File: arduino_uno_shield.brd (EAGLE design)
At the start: 53 x 59.7 mm, 18 parts

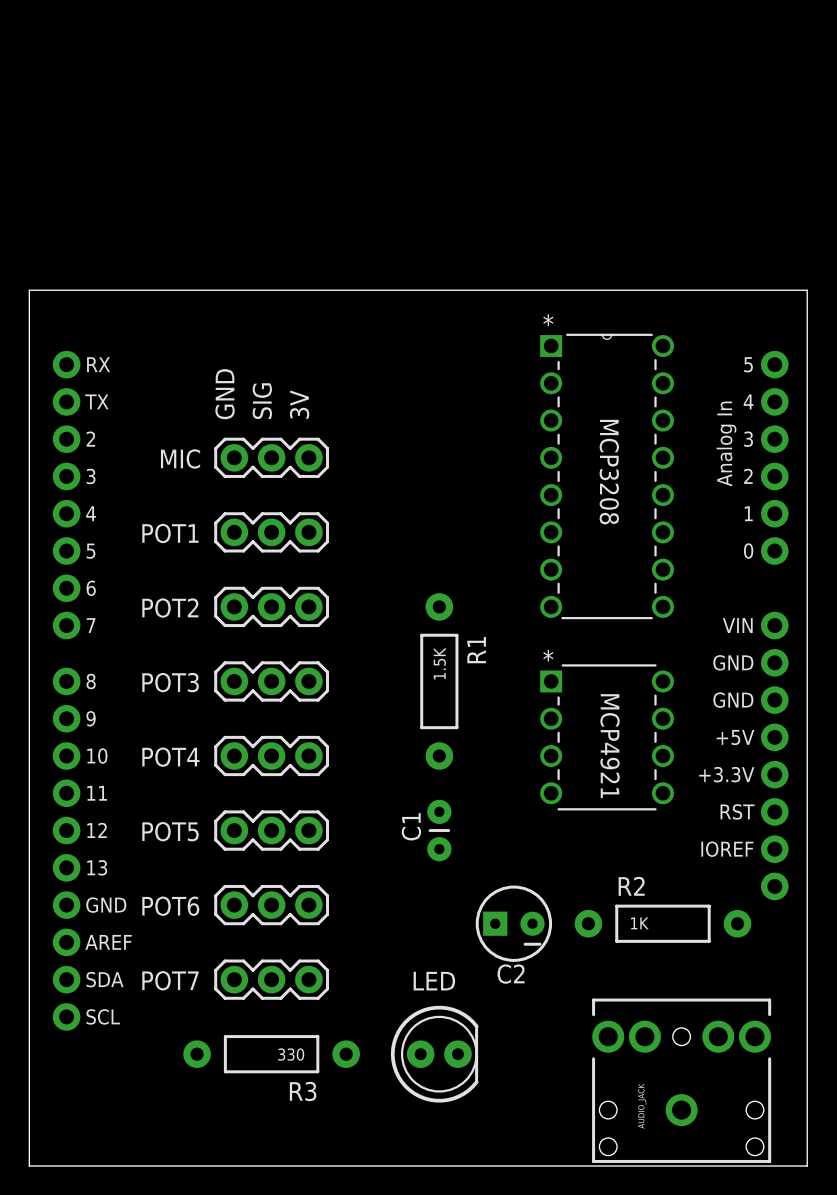
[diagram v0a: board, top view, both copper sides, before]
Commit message: created board from scratch
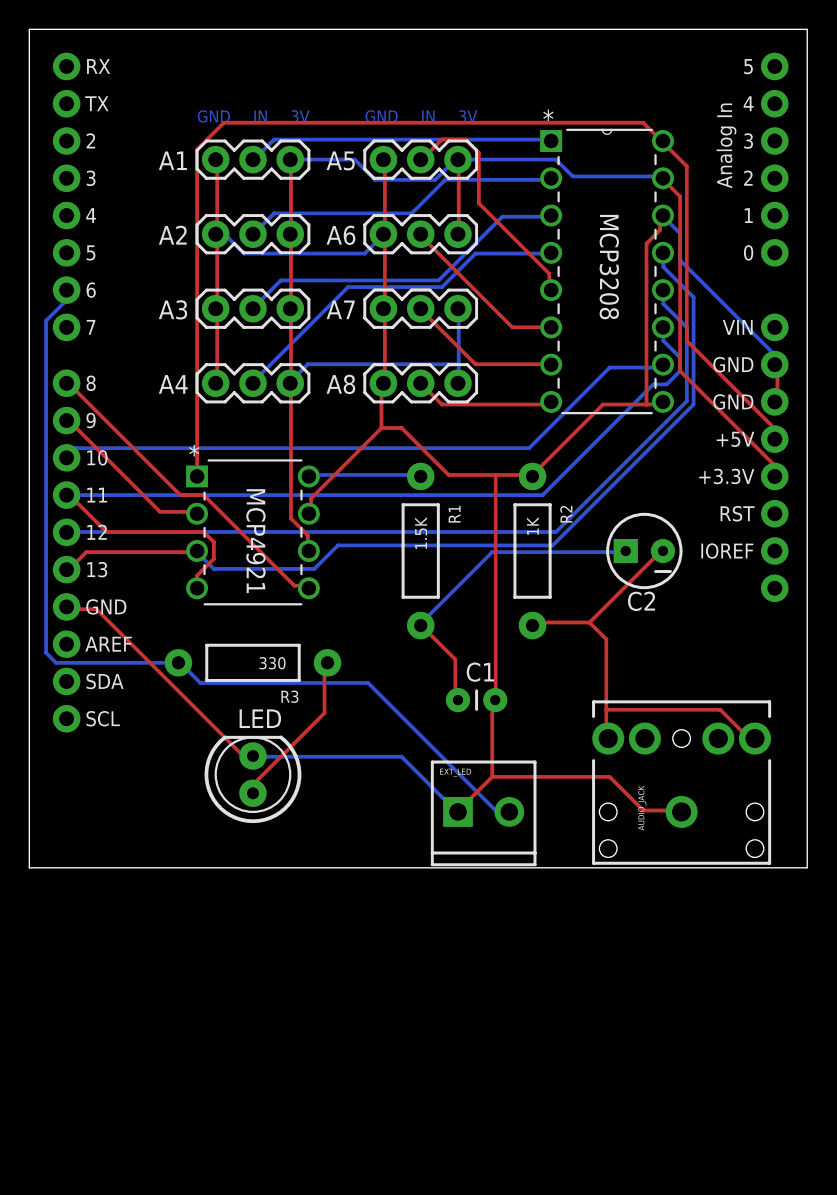
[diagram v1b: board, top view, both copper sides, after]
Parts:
- removed MIC, POT1, POT2, POT3, POT4, POT5, POT6, POT7: (no value), SparkFun-Connectors:1X03
- added A1, A2, A3, A4, A5, A6, A7, A8: (no value), SparkFun-Connectors:1X03
- added EXT_LED: M023.5MM, SparkFun-Connectors:SCREWTERMINAL-3.5MM-2
- moved MCP4921 27.9 mm to (19.1, 39.4)
- moved C2 26.9 mm to (41.9, 41.9)
- moved R2 26.9 mm to (34.3, 41.9), turned to 270 degrees
- moved R3 26.7 mm to (15.2, 34.3)
- moved LED 22.9 mm to (15.2, 26.7), turned to 90 degrees
- moved AUDIO_JACK 20.3 mm to (44.5, 24.1)
- moved U$1 20.3 mm to (0.00, 20.3)
- moved MCP3208 14.0 mm to (43.2, 52.1)
- moved C1 10.2 mm to (29.2, 31.8), turned to 0 degrees
- moved R1 8.98 mm to (26.7, 41.9)
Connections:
- net N$7 renamed A6
- net 3.3V: now also A1.3, A2.3, A3.3, A4.3, A5.3, A6.3, A7.3, A8.3; no longer MIC.3, POT1.3, POT2.3, POT3.3, POT4.3, POT5.3, POT6.3, POT7.3
- net AUD: now also A1.2; no longer MIC.2
- net GND: now also A1.1, A2.1, A3.1, A4.1, A5.1, A6.1, A7.1, A8.1, EXT_LED.1; no longer MIC.1, POT1.1, POT2.1, POT3.1, POT4.1, POT5.1, POT6.1, POT7.1
- net N$1: now also A5.2; no longer POT4.2
- net N$12: now also EXT_LED.2
- net N$14: now also A3.2; no longer POT2.2
- net N$15: now also A4.2; no longer POT3.2
- net N$16: now also A6.2; no longer POT5.2
- net N$17: now also A7.2; no longer POT6.2
- net N$18: now also A8.2; no longer POT7.2
- net N$2: now also A2.2; no longer POT1.2
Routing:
- net GND: track 0.00 -> 177.1 mm
- net 3.3V: track 0.00 -> 100.1 mm
- net 5V: track 0.00 -> 78.7 mm
- net A6: track 0.00 -> 63.8 mm
- net N$12: track 0.00 -> 61.4 mm
- net N$4: track 0.00 -> 59.7 mm
- net N$6: track 0.00 -> 54.2 mm
- net N$13: track 0.00 -> 43.3 mm
- net N$9: track 0.00 -> 30.5 mm
- net N$15: track 0.00 -> 24.0 mm
- net N$14: track 0.00 -> 22.9 mm
- net N$8: track 0.00 -> 22.4 mm
- net N$11: track 0.00 -> 22.3 mm
- net N$2: track 0.00 -> 21.9 mm
- net AUD: track 0.00 -> 20.9 mm
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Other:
- board size 53 x 59.7 mm -> 53 x 57.1 mm
- board text added: "IN"
- board text removed: "SIG"
